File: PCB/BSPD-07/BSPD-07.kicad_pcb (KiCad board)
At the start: 2 copper layers, 31.8 x 53.9 mm, 59 parts, among them IC1 LM393LVQDRQ1, IC2 LM393LVQDRQ1, IC3 LM393LVQDRQ1, IC4 LDO40LPU50RY, IC5 74LVC1G02GW-Q100H, J1 DTM13-12PA, Q1 RSQ025P03HZGTR, Q2 RJU002N06FRAT106, Q3 RJU002N06FRAT106, U2 TLP175A / COMUS AB38-Q

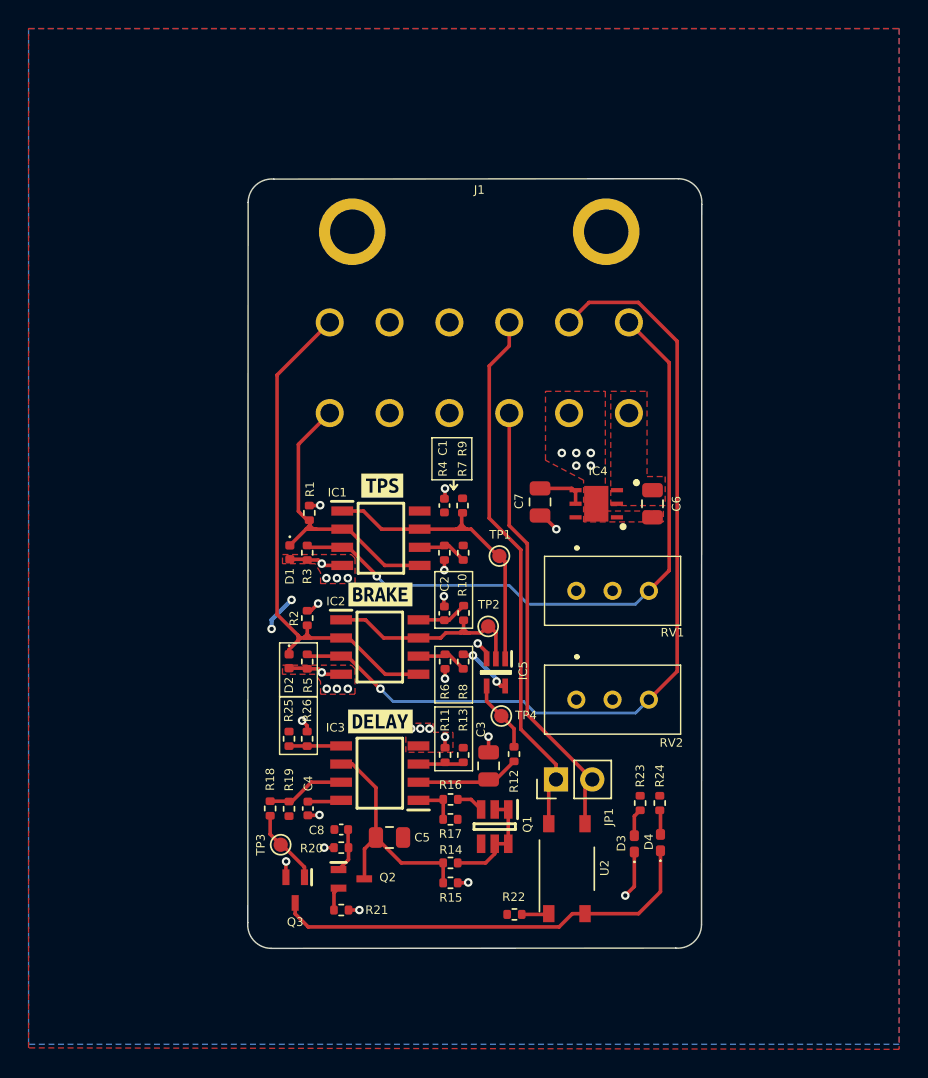
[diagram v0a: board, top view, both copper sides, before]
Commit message: Revised layout
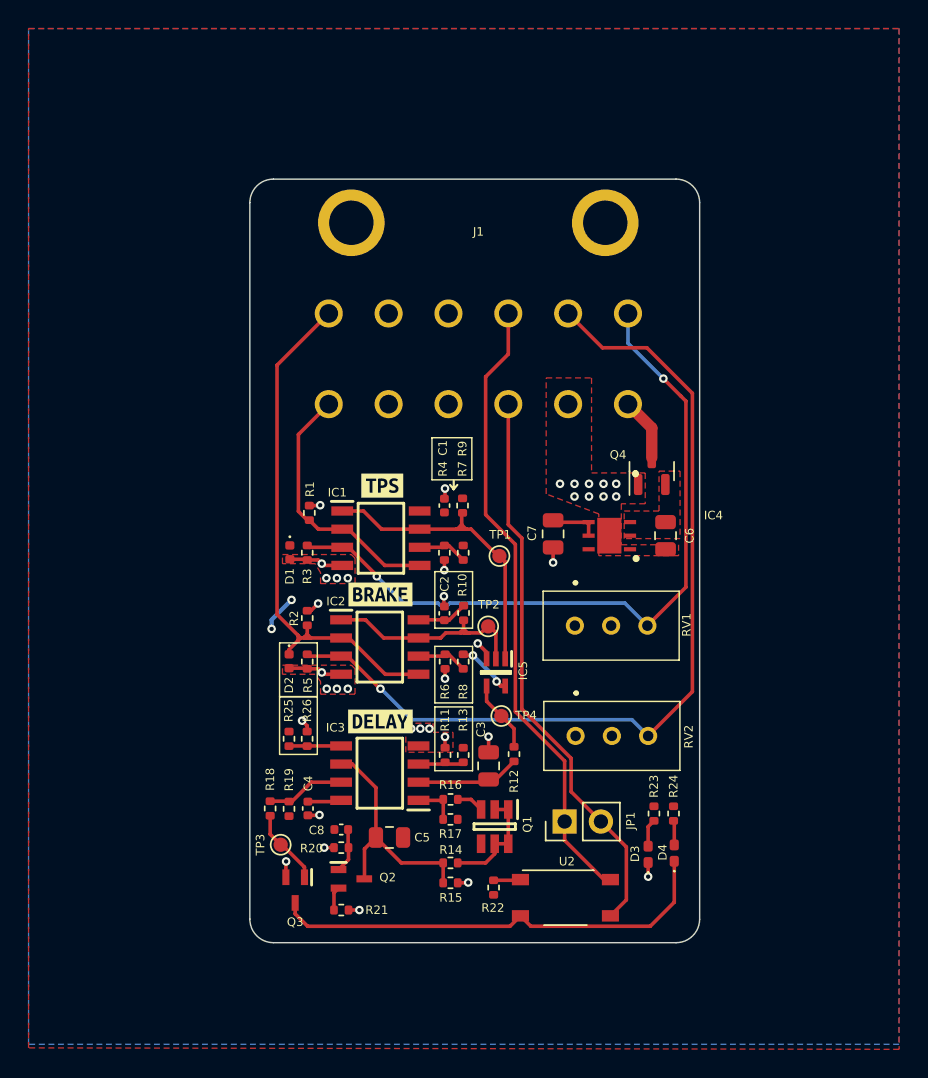
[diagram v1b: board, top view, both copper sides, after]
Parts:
- removed kibuzzard-64754545: G***, kibuzzard-64754545
- added Q4: AO3401A, Package_TO_SOT_SMD:SOT-23, F.Cu at (176.1, 102.9)
- added kibuzzard-647616BB: G***, kibuzzard-647616BB, F.Cu at (157.1, 111.5)
- moved JP1 3.01 mm to (170.0, 127.4)
- moved RV2 2.54 mm to (173.3, 121.4)
- moved RV1 2.44 mm to (173.2, 113.7)
- moved C6 2.42 mm to (177.0, 107.4)
- moved IC4 2.42 mm to (173.1, 107.4)
- moved C7 2.42 mm to (169.2, 107.3)
- moved R22 2.38 mm to (165.0, 132.1), turned to -90 degrees
- moved U2 2.03 mm to (170.0, 132.8), turned to 0 degrees
- moved D3 1.21 mm to (175.8, 129.7)
- moved D4 1.21 mm to (177.6, 129.6)
- moved R23 1.21 mm to (176.2, 126.9)
- moved R24 1.21 mm to (177.6, 126.9)
- moved J1 0.63 mm to (174.4, 98.2)
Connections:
- C6 pad 1: +12V -> Net-(C6-Pad1)
- IC4 pad 2: +12V -> Net-(C6-Pad1)
- IC4 pad 3: +12V -> Net-(C6-Pad1)
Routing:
- net SAFETY_OUT: track 31.4 -> 39.7 mm
- net SAFETY_IN: track 37.8 -> 44.2 mm
- net +12V: track 0.00 -> 4.44 mm
- net TPS_TRIG: track 46.6 -> 51.0 mm, vias 1 -> 2
- net GND: track 25.3 -> 22.5 mm, vias 33 -> 37
- net TPS_IN: track 20.9 -> 18.4 mm
- net BRAKE_TRIG: track 61.2 -> 62.5 mm
- net INFO_LED: track 30.6 -> 31.8 mm
- net BRAKE_IN: track 37.0 -> 37.6 mm
- added copper zone on F.Cu, net Net-(C6-Pad1)
- removed copper zone on F.Cu, net +12V
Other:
- board size 31.8 x 53.9 mm -> 31.5 x 53.5 mm
